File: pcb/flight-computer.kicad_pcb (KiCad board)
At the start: 4 copper layers, 83.7 x 62.9 mm, 90 parts, among them J1 MicroSD Slot, J2 USB_C_Receptacle_USB2.0_16P, J3 SMA_Coax, J4 Conn_01x02, J5 ARM, Q1 PMOS, U1 RP2040, U10 LM3671MF, U11 TPS2116DRL, U2 W25Q16JVSS, U3 USBLC6-2SC6, U4 M24C32-FMN, U5 MS5607-02BA, U6 LIS2MDL, U7 LSM6DSO32TR, U8 LC86G, U9 RN2903, Y1 12MHz

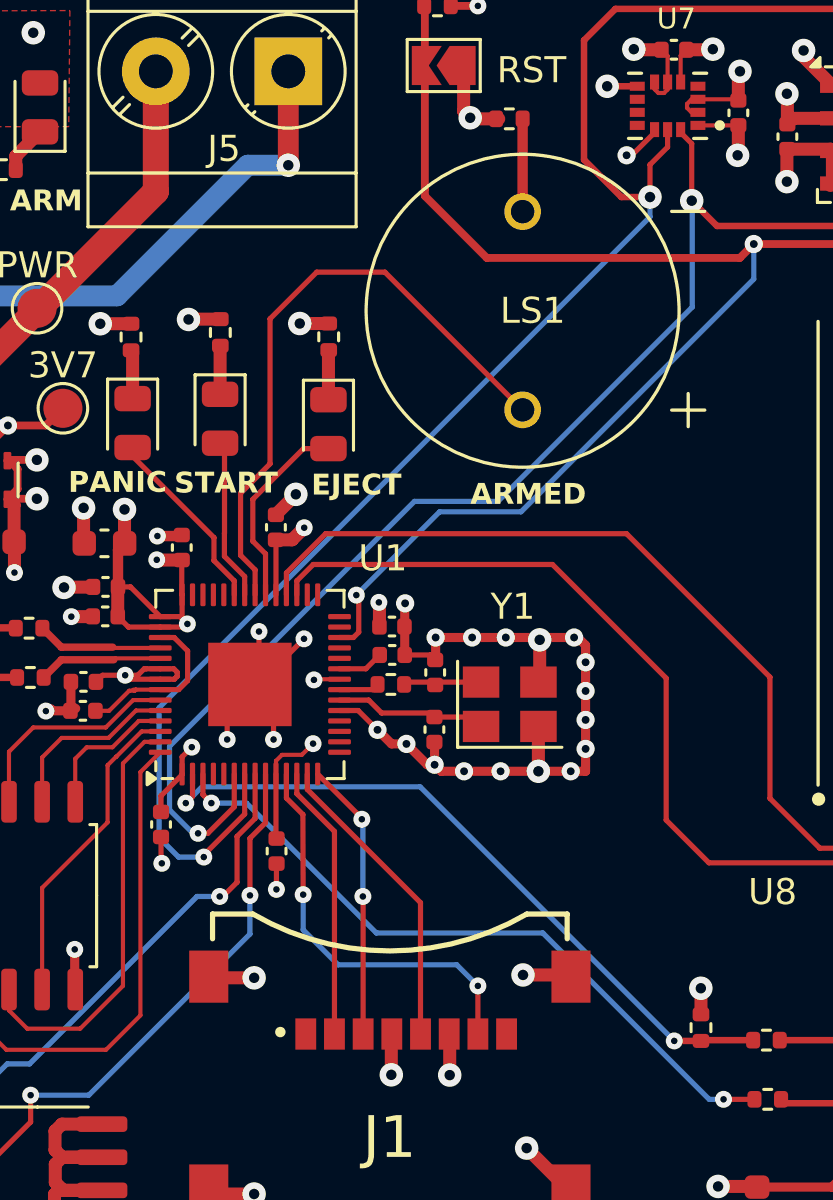
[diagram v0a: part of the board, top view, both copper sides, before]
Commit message: Teardrops and some cleanup
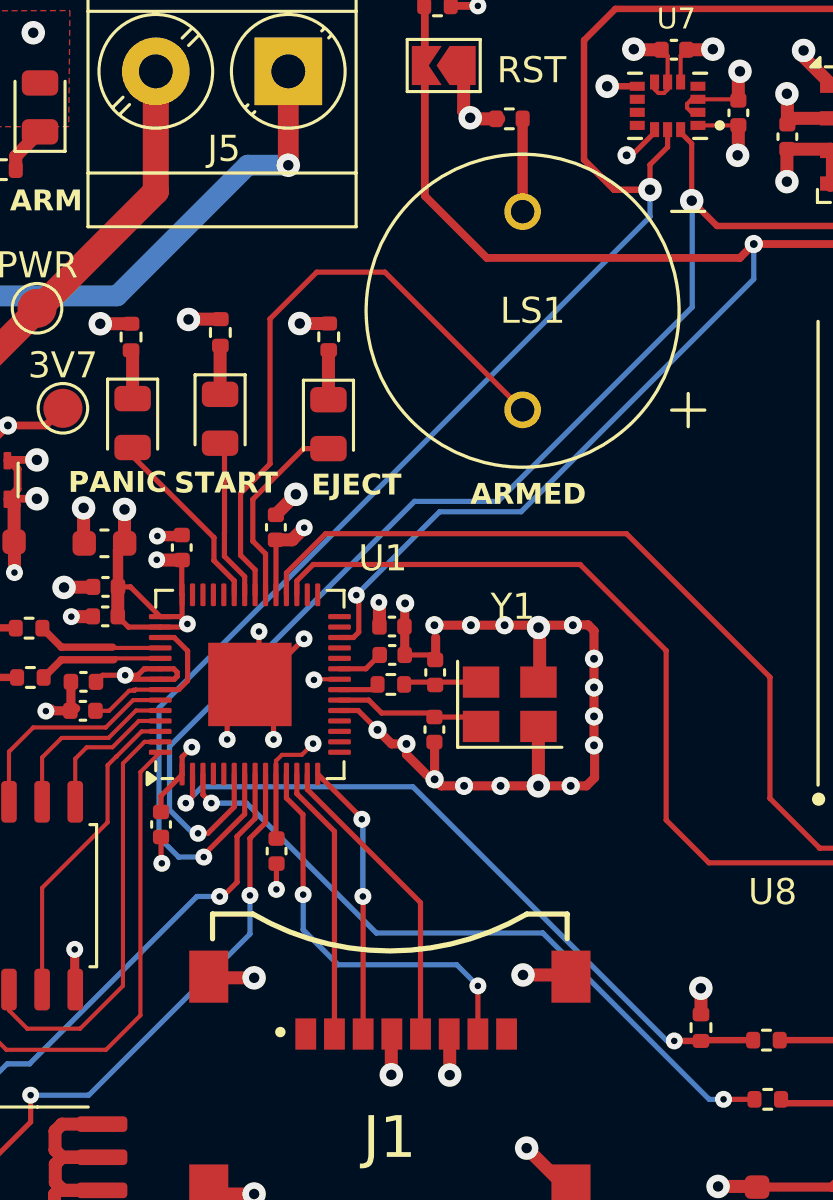
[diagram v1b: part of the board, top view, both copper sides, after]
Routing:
- net GND: track 297.5 -> 300.3 mm
- net MCU_UART1_TX: track 39.6 -> 40.2 mm
